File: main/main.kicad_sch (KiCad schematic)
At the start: 20 parts, among them SW6 RotaryEncoder, U1 STM32F411CEU6, U100 AP1117-33, U4 AT24CS64-SSHM, Y1 32768kHz

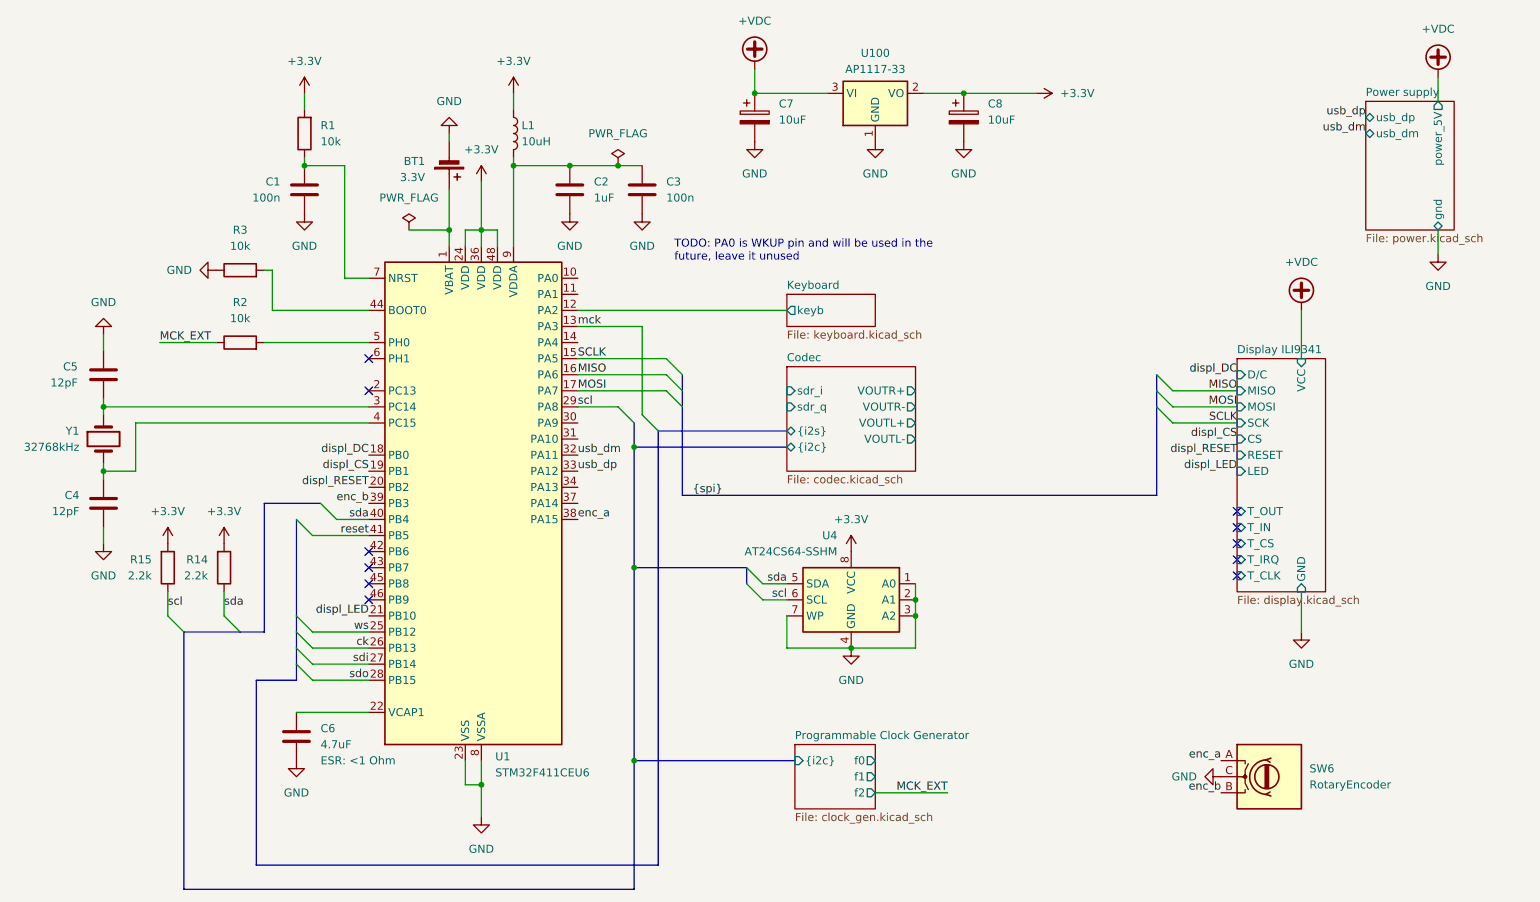
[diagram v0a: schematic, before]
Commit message: Key added
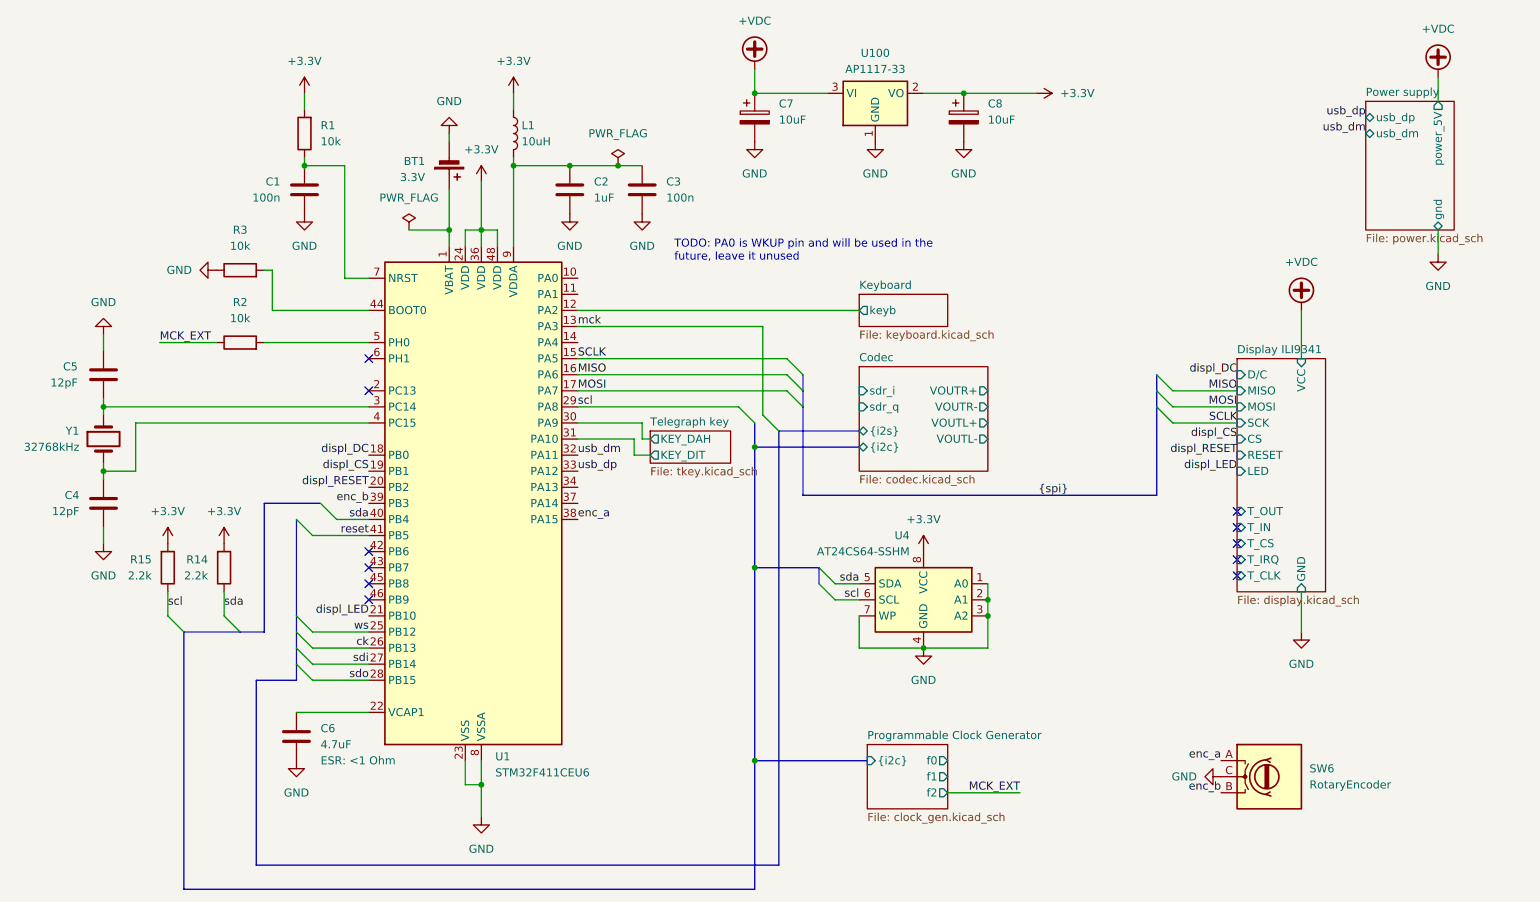
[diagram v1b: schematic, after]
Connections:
- net Telegraph key/KEY_DAH: now reaches U1.30 (PA9)
- net Telegraph key/KEY_DIT: now reaches U1.31 (PA10)
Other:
- added sheet Telegraph key (tkey.kicad_sch)
- moved on the sheet: U4
